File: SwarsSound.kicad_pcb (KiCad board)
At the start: 2 copper layers, 292.1 x 227.3 mm, 168 parts, among them P1 Main_Connector, P2 aud_con, P3 edge_con, Q1 2N3906f, Q2 2N3906f, Q3 2N3904, Q4 2N3904

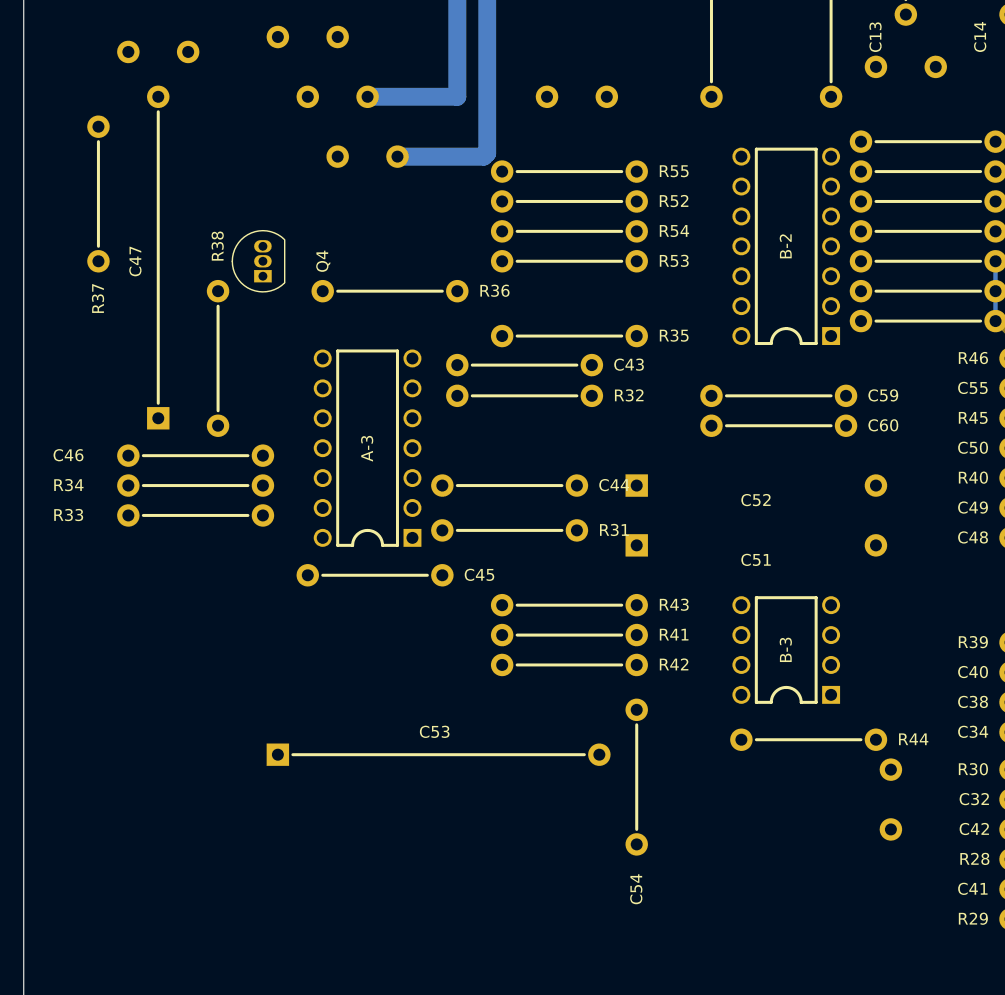
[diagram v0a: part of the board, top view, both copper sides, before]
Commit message: more traces
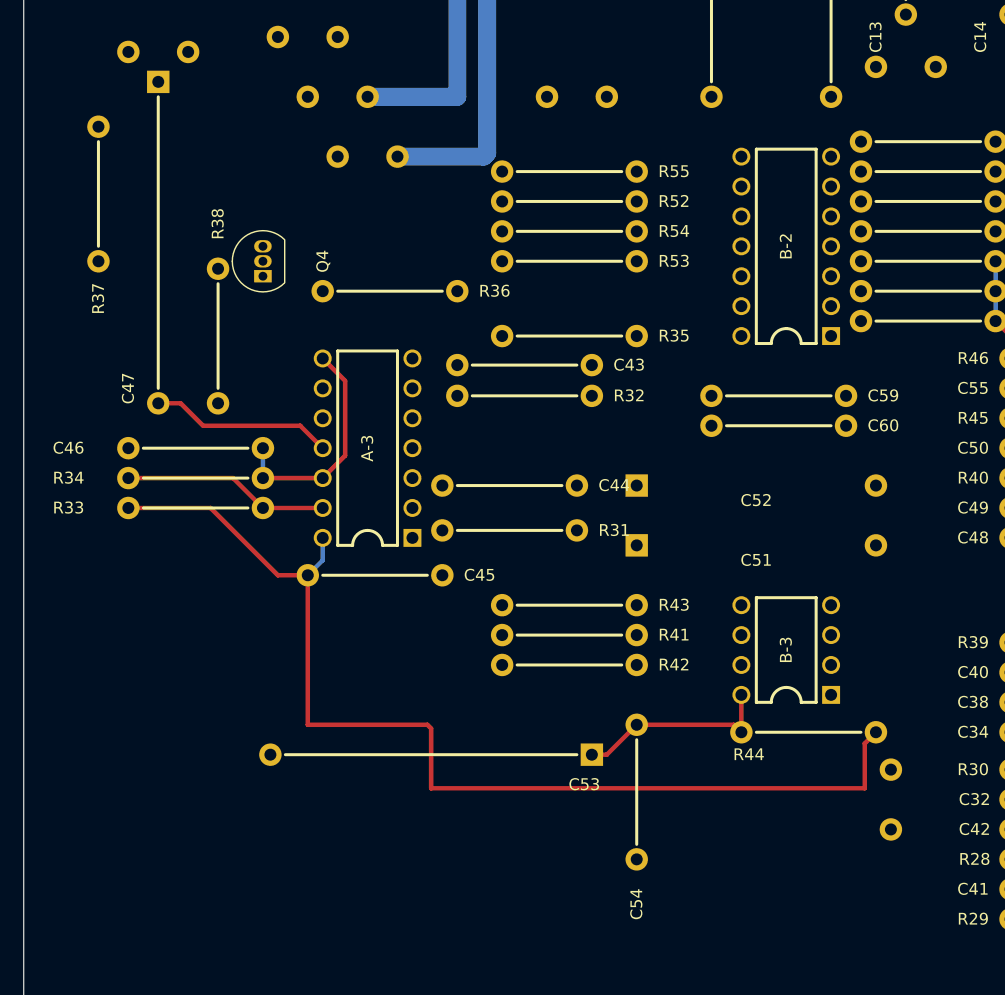
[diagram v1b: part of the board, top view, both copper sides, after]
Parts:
- moved C47 1.91 mm to (29.2, 111.1), turned to 270 degrees
- moved R38 1.91 mm to (34.3, 120.0)
- moved R34 1.42 mm to (33.0, 131.4), turned to 90 degrees
- moved R44 1.42 mm to (85.1, 153.0), turned to 90 degrees
- moved R33 1.42 mm to (33.0, 134.0), turned to 90 degrees
- moved C46 0.63 mm to (31.8, 128.9)
- turned C53 to 180 degrees
- turned C54 to 180 degrees
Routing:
- net +12V: track 120.8 -> 211.8 mm
- net Net-(A-3-Pad12): track 0.00 -> 19.4 mm
- net Net-(A-3-Pad13): track 0.00 -> 17.6 mm
- net Net-(B-3-Pad8): track 0.00 -> 17.2 mm
- net Net-(A-3-Pad11): track 0.00 -> 15.5 mm
